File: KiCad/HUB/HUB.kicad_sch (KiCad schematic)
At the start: 11 parts, among them IC1 AT32UC3B164-AUT, J1 ESP8266(wifi), J2 USB_B_Mini, SW1 SW_MEC_5E, SW2 SW_MEC_5E, SW3 SW_MEC_5E

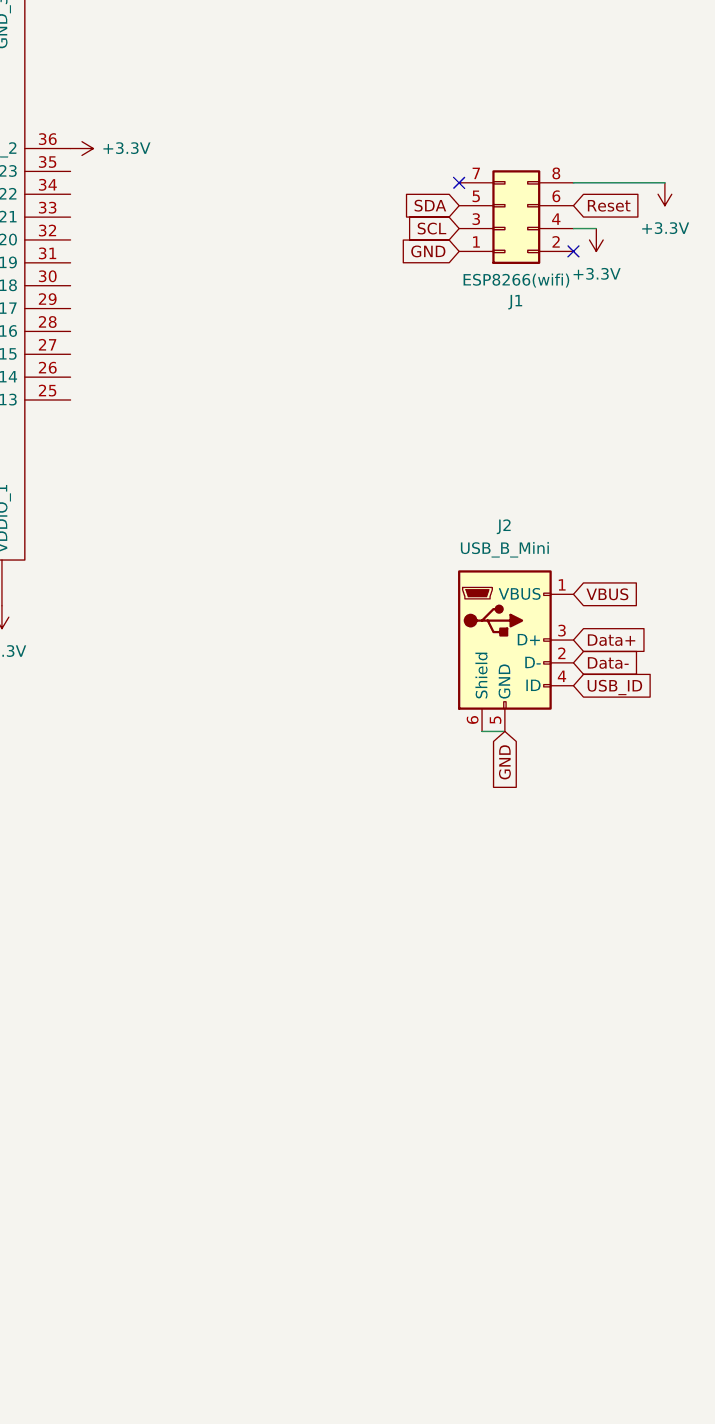
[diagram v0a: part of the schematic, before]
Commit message: hub
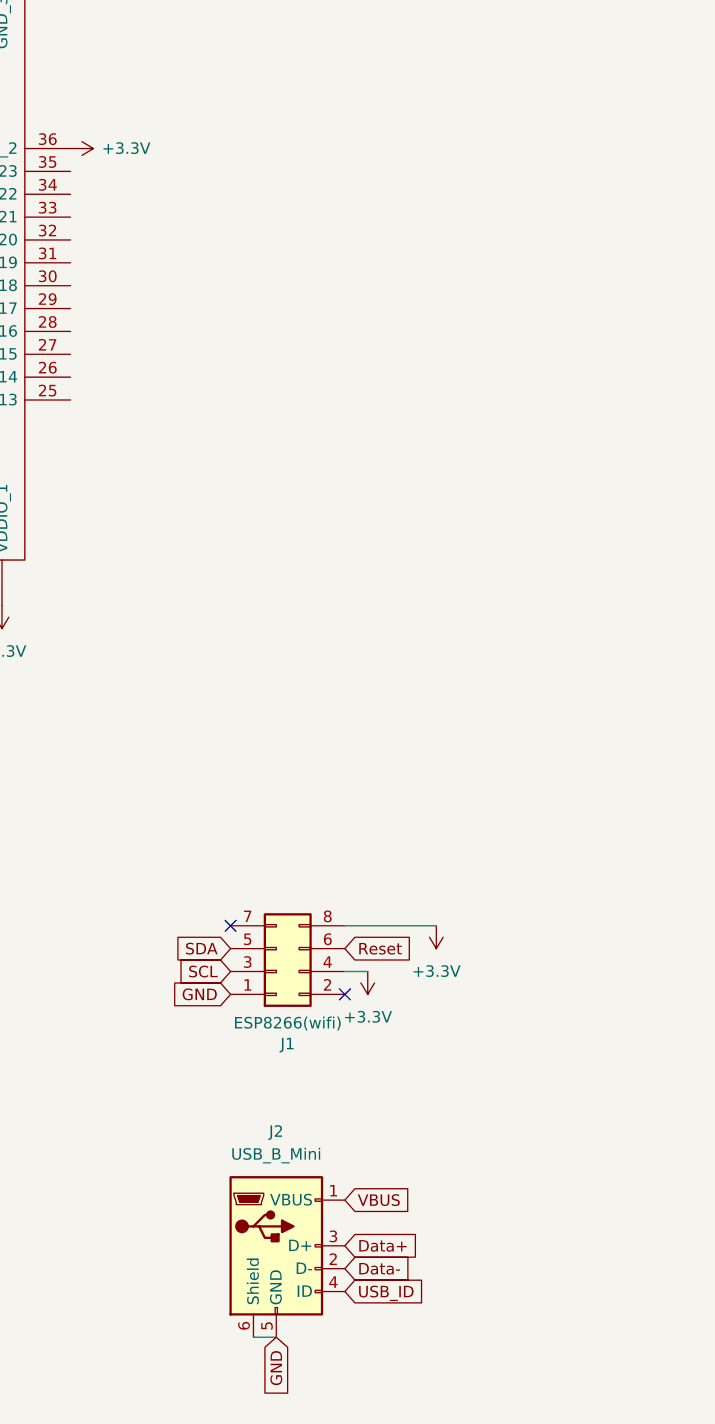
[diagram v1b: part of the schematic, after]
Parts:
- IC1: footprint (none) -> user:QFP50P900X900X120-48N
- J2: footprint (none) -> Connector_USB:USB_Mini-B_Lumberg_2486_01_Horizontal
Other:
- moved on the sheet: J1, J2
